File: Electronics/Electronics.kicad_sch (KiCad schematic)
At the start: 14 parts, among them P1 USB_C_Plug_USB2.0, SW5 SW_DIP_x02, U11 AMS1117-3.3, U12 AMS1117-3.3

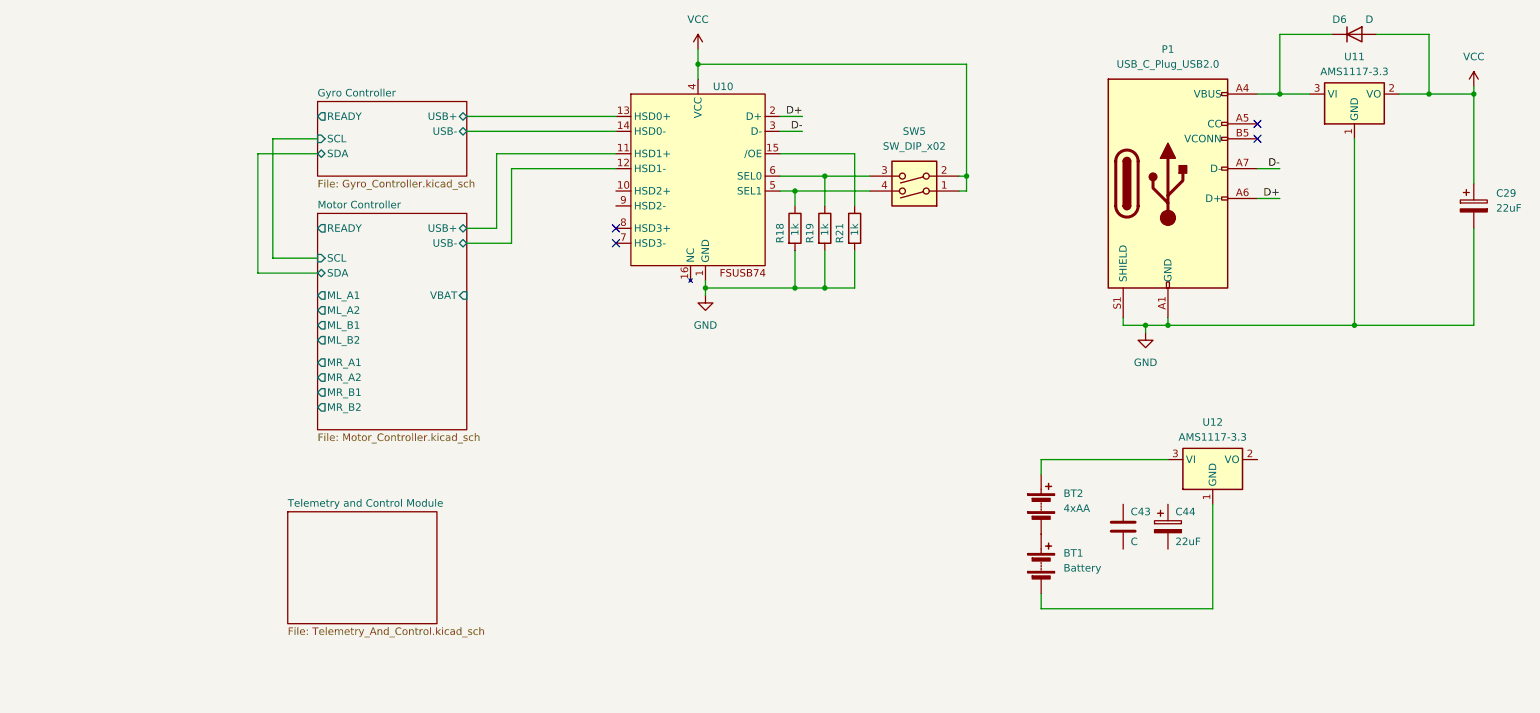
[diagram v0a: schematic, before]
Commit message: mostly done, needs review, needs pins
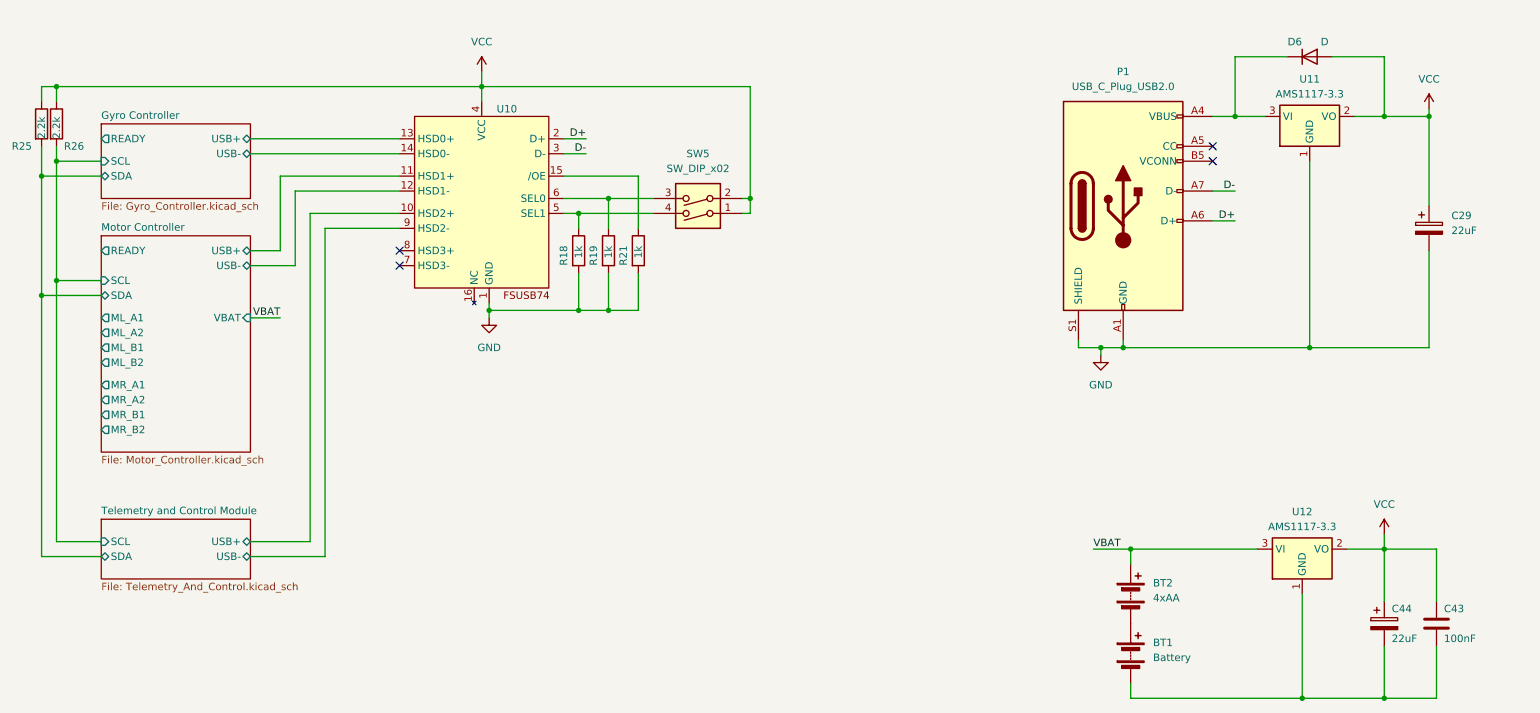
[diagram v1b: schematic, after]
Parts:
- added R25, R26: 2.2k, symbol Device:R
- C43: value C -> 100nF
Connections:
- net Gyro Controller/SCL: now also R26.2
- net Gyro Controller/SDA: now also R25.2
- net VCC: now also C43.1, C44.1, U12.2 (VO), R25.1, R26.1
- net at C44.2: now also BT1.2 (-), C43.2, U12.1 (GND)
- net VBAT: now reaches BT2.1 (+), U12.3 (VI)
- net Telemetry and Control Module/USB+: now reaches U10.10 (HSD2+)
- net Telemetry and Control Module/USB-: now reaches U10.9 (HSD2-)
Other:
- sheet Telemetry and Control Module ports: added SCL, SDA, USB+, USB-; removed none
- moved on the sheet: BT1, BT2, C29, C43, C44, D6, P1, R18, R19, R21, SW5, U10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
